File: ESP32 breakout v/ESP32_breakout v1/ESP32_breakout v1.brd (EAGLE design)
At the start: 100 x 80 mm, 25 parts, among them U1 ESP-WROOM-32, U2 AP7361C-33E-13

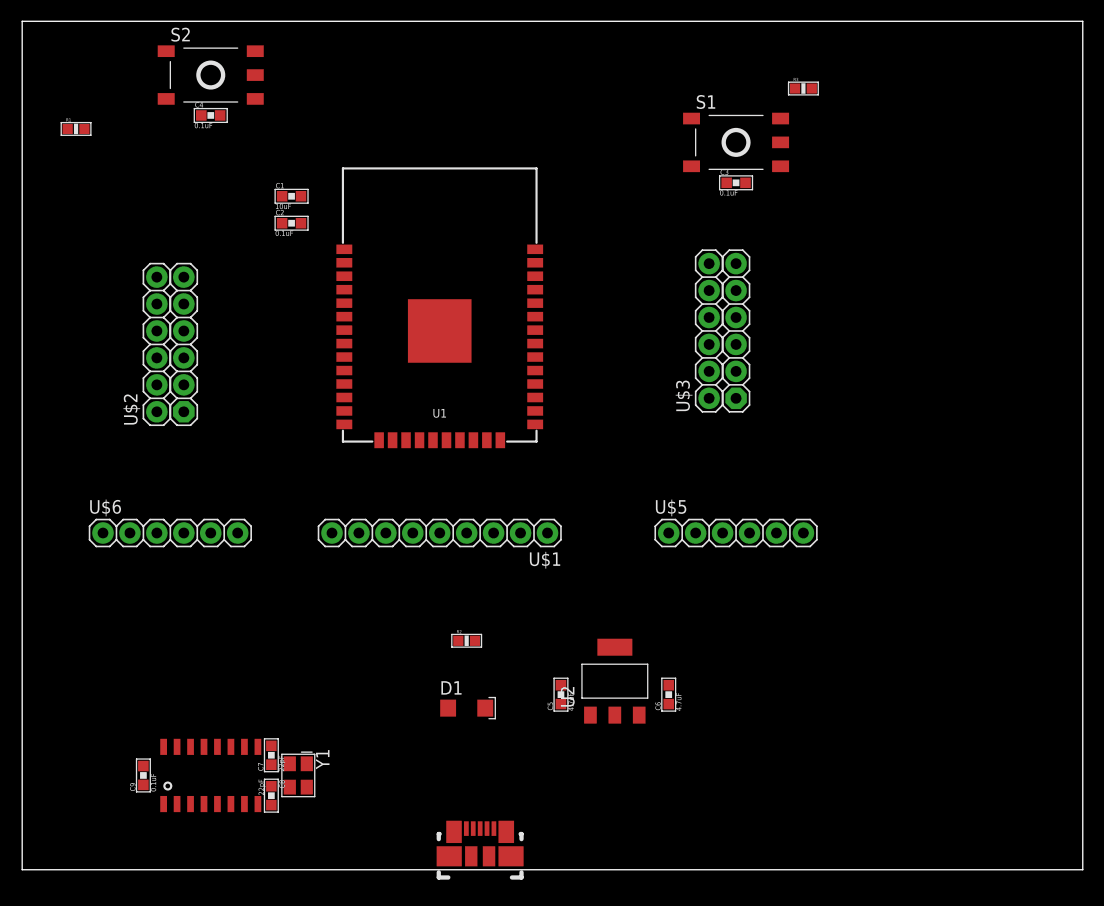
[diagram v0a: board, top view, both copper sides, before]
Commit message: layout
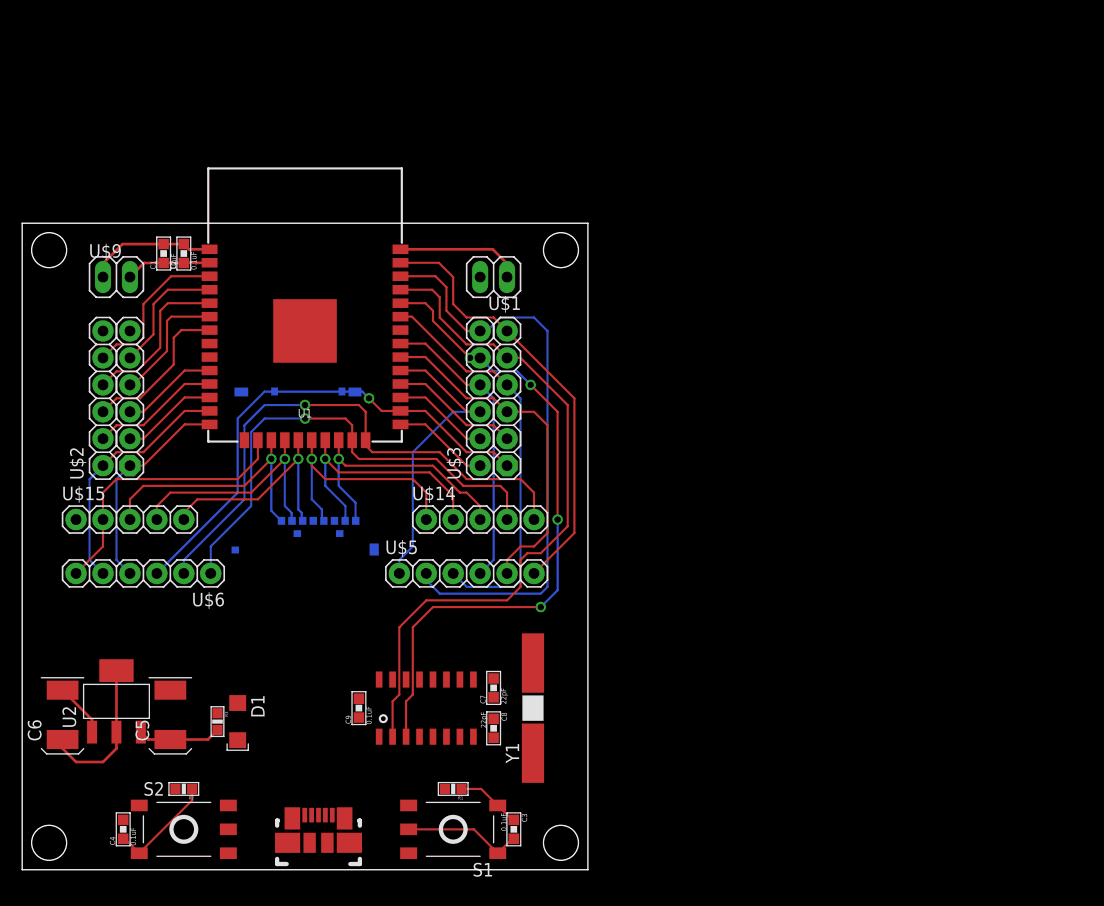
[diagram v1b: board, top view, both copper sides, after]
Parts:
- added U$10, U$11, U$12, U$13: (no value), EmbeddedAdventures 3:STAND-OFF-HOLE
- added U$14, U$15: M05, dr-library:1X05
- added U$8: SCHA4B0419, dr-library:MICROSD_SCHA4B0419
- added U$9: M02LONG, dr-library:1X02-LONG
- C5, C6: value 4.7uF -> 10uF; device dr-library:CAP-0603 -> dr-library:B-3528
- U$1: value M09 -> M02LONG; device dr-library:1X09 -> dr-library:1X02-LONG
- U2: value AP7361C-33E-13 -> (none); device dr-library:SOT-223-3 -> dr-library:SOT-223-4
- Y1: value (none) -> 12MHz; device dr-library:CFPX-180 -> dr-library:HC-49/US
- moved R3 81.3 mm to (18.4, 14.0), turned to 270 degrees
- moved R1 71.7 mm to (40.6, 7.62), turned to 180 degrees
- moved S2 71.2 mm to (15.2, 3.81)
- moved S1 70.0 mm to (40.6, 3.81), turned to 180 degrees
- moved C4 67.8 mm to (9.53, 3.81), turned to 90 degrees
- moved C3 64.5 mm to (46.4, 3.81), turned to 270 degrees
- moved C6 57.2 mm to (3.81, 14.6)
- moved U2 47.0 mm to (8.89, 15.9)
- moved C5 36.9 mm to (14.0, 14.6)
- moved R2 30.1 mm to (15.2, 7.62), turned to 180 degrees
- moved U$5 25.7 mm to (36.8, 27.9)
- moved U$1 24.4 mm to (44.5, 55.9)
- moved Y1 23.1 mm to (48.3, 15.2), turned to 90 degrees
- moved U$3 22.5 mm to (43.2, 39.4)
- moved C7 21.9 mm to (44.5, 17.1)
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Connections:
- net +3V3: now also C6.P, U$8.4, U$9.2, U2.2, U2.PAD; no longer C6.1, U2.3
- net CLK: now also U$14.1, U$8.5; no longer U$1.5
- net CMD: now also U$15.5, U$8.3; no longer U$1.6
- net GND: now also C5.N, C6.N, U$1.1, U$15.1, U$8.6, U$8.G1, U$8.G2, U$9.1, U2.1; no longer C5.2, C6.2, U2.2, Y1.2, Y1.4
- net IO0: now also U$3.2; no longer U$3.1
- net IO13: now also U$15.2; no longer U$1.9
- net IO15: now also U$14.4; no longer U$1.2
- net IO16: now also U$3.4; no longer U$3.3
- net IO17: now also U$3.3; no longer U$3.4
- net IO18: now also U$3.5; no longer U$3.6
- net IO19: now also U$3.8; no longer U$3.7
- net IO2: now also U$14.5; no longer U$1.1
- net IO21: now also U$3.7; no longer U$3.8
- net IO22: now also U$3.12; no longer U$3.11
- net IO23: now also U$3.11; no longer U$3.12
- net IO4: now also U$3.1; no longer U$3.2
- net IO5: now also U$3.6; no longer U$3.5
- net N$3: now also Y1.P$1; no longer Y1.1
- net N$4: now also Y1.P$2; no longer Y1.3
- net RX: now also U$3.10; no longer U$3.9
- net SD0: now also U$14.2, U$8.7; no longer U$1.4
- net SD1: now also U$14.3, U$8.8; no longer U$1.3
- net SD2: now also U$15.3, U$8.1; no longer U$1.8
- net SD3: now also U$15.4, U$8.2; no longer U$1.7
- net TX: now also U$3.9; no longer U$3.10
- net VCC: now also C5.P, U$1.2, U2.3; no longer C5.1, U2.1
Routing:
- net TX: track 0.00 -> 64.7 mm
- net RX: track 0.00 -> 63.1 mm, vias 0 -> 4
- net IO22: track 0.00 -> 55.3 mm
- net IO2: track 0.00 -> 52.3 mm, vias 0 -> 1
- net IO4: track 0.00 -> 47.1 mm, vias 0 -> 1
- net IO15: track 0.00 -> 46.5 mm, vias 0 -> 1
- net IO23: track 0.00 -> 41.3 mm
- net GND: track 0.00 -> 40.7 mm
- net IO21: track 0.00 -> 38.8 mm
- net IO18: track 0.00 -> 32.8 mm
- net IO5: track 0.00 -> 29.0 mm
- net IO19: track 0.00 -> 28.0 mm
- net IO13: track 0.00 -> 26.4 mm
- net SD2: track 0.00 -> 24.8 mm, vias 0 -> 1
- net SD1: track 0.00 -> 24.7 mm, vias 0 -> 1
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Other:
- board size 100 x 80 mm -> 53.3 x 61 mm
